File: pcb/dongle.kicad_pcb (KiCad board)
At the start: 2 copper layers, 14 x 20 mm, 29 parts, among them J1 USB_A, J2 Conn_01x01_Pin, J3 Conn_01x01_Pin, J4 Conn_01x01_Pin, J5 Conn_01x01_Pin, SW1 SW_Push_45deg, U3 nRF52833_QDxx, Y1 Crystal_GND24, Y2 Crystal_Small

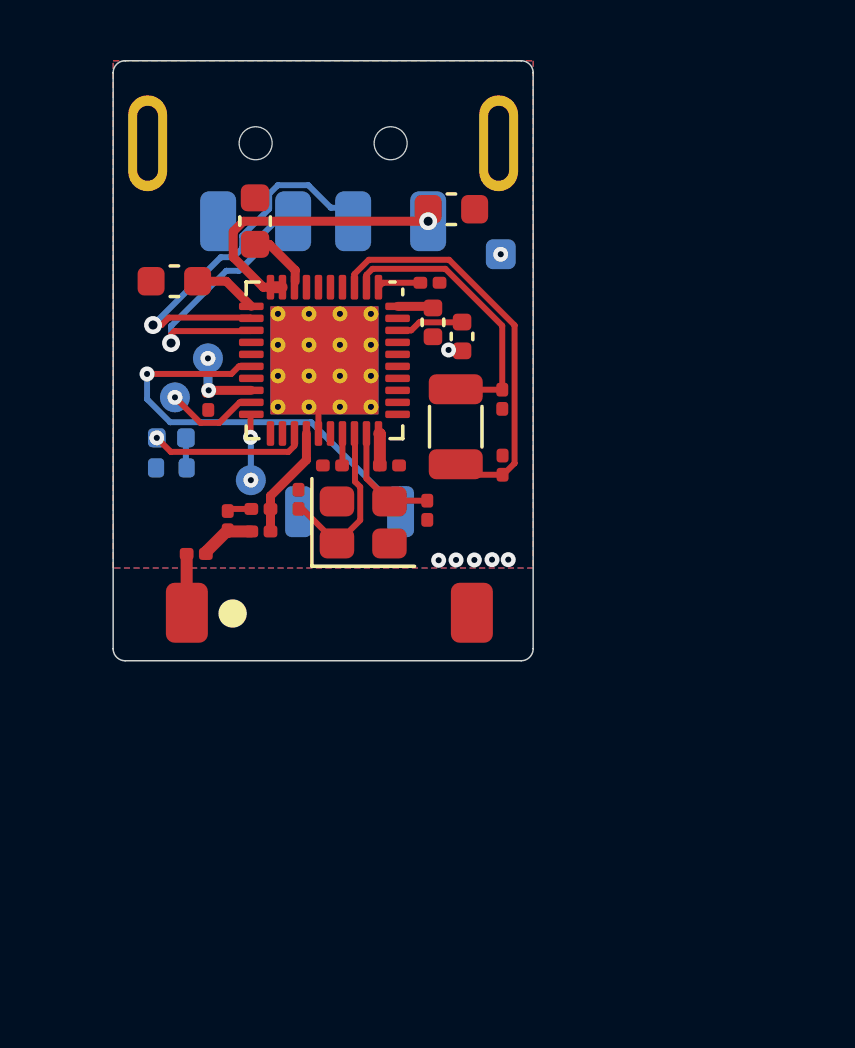
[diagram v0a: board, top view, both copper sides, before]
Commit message: clear pcb
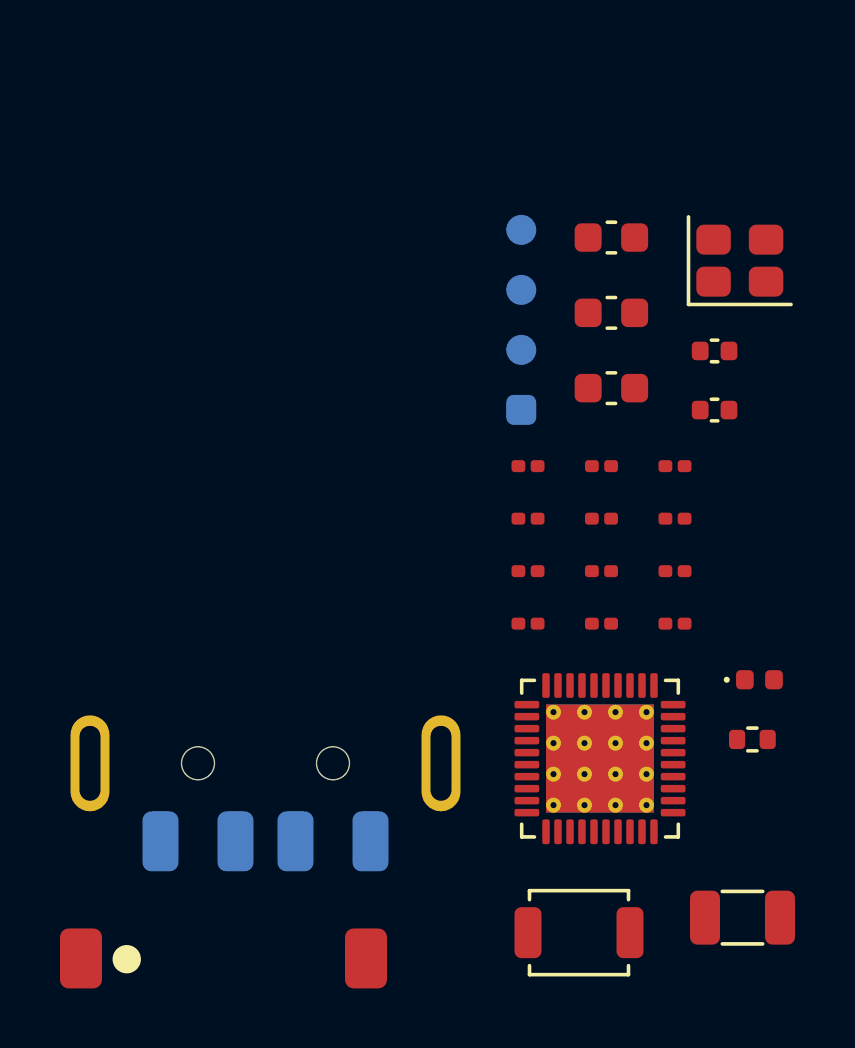
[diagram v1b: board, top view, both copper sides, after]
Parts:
- D1, R1, SW1: moved to F.Cu
- moved R1 21.4 mm to (160.1, 116.5), turned to 0 degrees
- moved D1 21.2 mm to (160.3, 114.5), turned to 0 degrees
- moved J1 20.8 mm to (143.7, 109.9)
- moved Y2 19.0 mm to (159.7, 122.5), turned to 0 degrees
- moved U3 16.1 mm to (155.0, 117.2), turned to 0 degrees
- moved L2 16.1 mm to (157.5, 112.7), turned to 0 degrees
- moved SW1 16.0 mm to (154.3, 123.0), turned to 0 degrees
- moved Y1 15.3 mm to (159.6, 100.6)
- moved C19 15.0 mm to (155.3, 104.8)
- moved L1 13.9 mm to (157.5, 110.9), turned to 0 degrees
- moved C7 13.7 mm to (155.0, 109.2), turned to 0 degrees
- moved AE1 12.1 mm to (140.5, 123.8)
- moved C6 11.9 mm to (155.3, 99.8), turned to 0 degrees
- moved J4 11.7 mm to (152.3, 103.5)
- moved J2 11.3 mm to (152.3, 99.5)
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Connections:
- C1 pad 1: VSS -> GND
- C10 pad 1: VSS -> GND
- C11 pad 1: VSS -> GND
- C12 pad 1: VSS -> GND
- C13 pad 1: VSS -> GND
- C15 pad 2: VSS -> GND
- C16 pad 1: VSS -> GND
- C17 pad 1: VSS -> GND
- C19 pad 1: VSS -> GND
- C2 pad 1: VSS -> GND
- C3 pad 1: VSS -> VSS_PA
- C4 pad 2: VSS -> GND
- C5 pad 1: VSS -> GND
- C6 pad 1: VSS -> GND
- C7 pad 1: VSS -> GND
- J1 pad 4: VSS -> GND
- J1 pad 5: VSS -> GND
- J5 pad 1: VSS -> GND
- R1 pad 2: VSS -> GND
- SW1 pad 2: VSS -> GND
- U3 pad 25: VSS -> VSS_PA
- U3 pad 37: VSS -> GND
- U3 pad 41: VSS -> GND
- Y1 pad 2: VSS -> GND
- Y1 pad 4: VSS -> GND
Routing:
- net RESET: track 14.4 -> 0.00 mm, vias 1 -> 0
- net XL2: track 13.7 -> 0.00 mm
- net D-: track 13.0 -> 0.00 mm, vias 1 -> 0
- net VBUS: track 9.92 -> 0.00 mm, vias 1 -> 0
- net XL1: track 9.50 -> 0.00 mm
- net D+: track 9.35 -> 0.00 mm, vias 1 -> 0
- net VDD: track 6.94 -> 0.00 mm, vias 2 -> 0
- net XC1: track 5.82 -> 0.00 mm
- net LED: track 5.28 -> 0.00 mm, vias 1 -> 0
- net XC2: track 3.85 -> 0.00 mm
- net ANT: track 3.76 -> 0.00 mm
- net VSS: track 3.33 -> 0.00 mm, vias 7 -> 0
- net SWD: track 3.18 -> 0.00 mm, vias 1 -> 0
- net DEC4: track 2.26 -> 0.00 mm
- net SWC: track 2.21 -> 0.00 mm, vias 2 -> 0
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- removed copper zone on B.Cu, net VSS
- removed copper zone on F.Cu, net VSS
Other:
- board outline removed
- board text removed: "SWC"
- board text removed: "SWD"
- board text removed: "VDD"
- board text removed: "VSS"
